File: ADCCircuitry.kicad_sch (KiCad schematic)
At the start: 26 parts, among them J1 Screw_Terminal_01x04, J2 Screw_Terminal_01x02, U2 ADS112C04, U3 ADS112C04, U4 ADS112C04, U5 ADS112C04

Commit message: v0.1 sch. Add devkit c1 footprint
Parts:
- J2: footprint (none) -> TerminalBlock:TerminalBlock_Xinya_XY308-2.54-2P_1x02_P2.54mm_Horizontal
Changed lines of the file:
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@@
 			)
 		)
-		(property "Footprint" ""
+		(property "Footprint" "TerminalBlock:TerminalBlock_Xinya_XY308-2.54-2P_1x02_P2.54mm_Horizontal"
 			(at 116.84 41.91 0)
 			(effects

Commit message: Add all footprints
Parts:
- U2, U3, U4, U5: footprint ADS112C04IPWR:SOP65P640X120-16N -> Package_SO:TSSOP-16_4.4x5mm_P0.65mm
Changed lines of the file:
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@@
 			)
 		)
-		(property "Footprint" "ADS112C04IPWR:SOP65P640X120-16N"
+		(property "Footprint" "Package_SO:TSSOP-16_4.4x5mm_P0.65mm"
 			(at 223.52 128.27 0)
 			(effects
@@
 			)
 		)
-		(property "Footprint" "ADS112C04IPWR:SOP65P640X120-16N"
+		(property "Footprint" "Package_SO:TSSOP-16_4.4x5mm_P0.65mm"
 			(at 223.52 77.47 0)
 			(effects
@@
 			)
 		)
-		(property "Footprint" "ADS112C04IPWR:SOP65P640X120-16N"
+		(property "Footprint" "Package_SO:TSSOP-16_4.4x5mm_P0.65mm"
 			(at 345.44 77.47 0)
 			(effects
@@
 			)
 		)
-		(property "Footprint" "ADS112C04IPWR:SOP65P640X120-16N"
+		(property "Footprint" "Package_SO:TSSOP-16_4.4x5mm_P0.65mm"
 			(at 345.44 128.27 0)
 			(effects

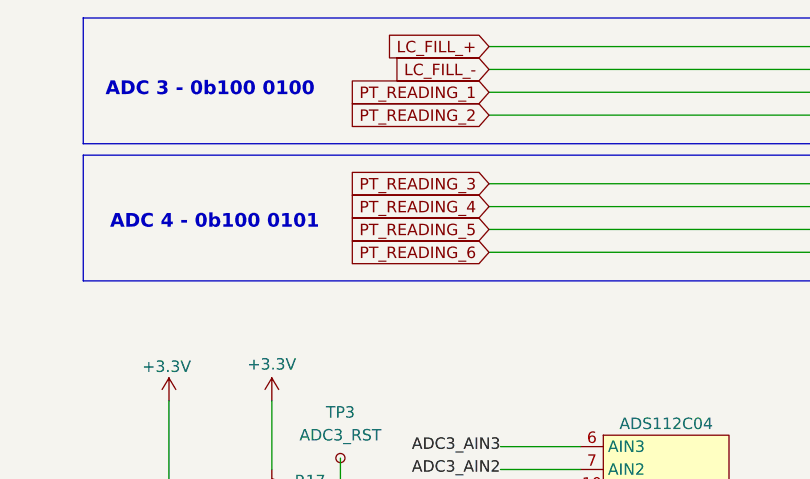
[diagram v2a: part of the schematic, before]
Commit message: Almost done routing
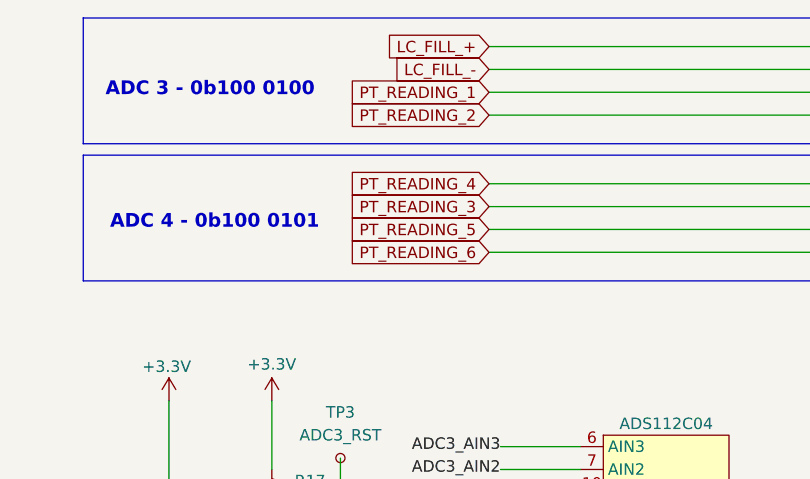
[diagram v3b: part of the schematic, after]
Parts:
- TP1, TP2, TP3, TP4: footprint TestPoint:TestPoint_Pad_D2.0mm -> TestPoint:TestPoint_Pad_D1.0mm
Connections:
- net PT_READING_3: now also U5.7 (AIN2); no longer U5.6 (AIN3)
- net PT_READING_4: now also U5.6 (AIN3); no longer U5.7 (AIN2)
